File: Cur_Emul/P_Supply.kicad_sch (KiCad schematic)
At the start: 47 parts, among them J31 Conn_01x02_Pin, J49 Conn_01x04_Pin, J50 Conn_01x04_Pin, J51 Conn_01x02_Pin, J52 Conn_01x02_Pin, J53 Conn_01x02_Pin, J54 Conn_01x02_Pin, J55 Conn_01x02_Pin, U13 LM317_SOT-223, U15 LM7812_TO220, U7 LM317_SOT-223

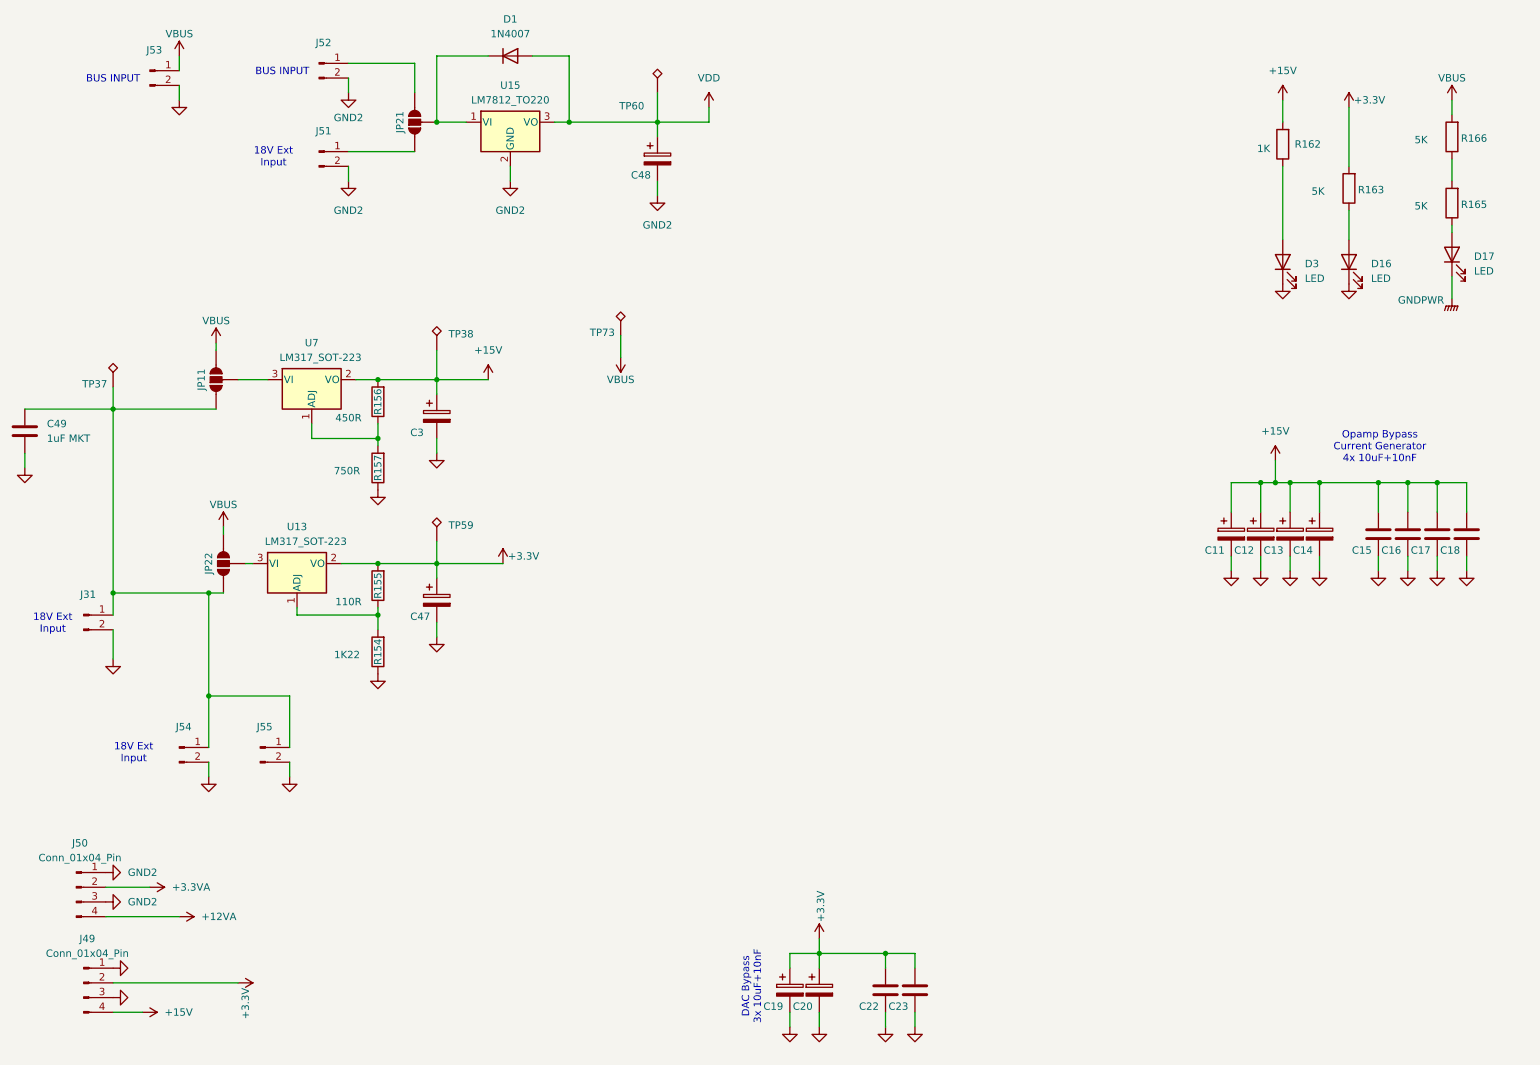
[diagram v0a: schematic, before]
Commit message: updates4
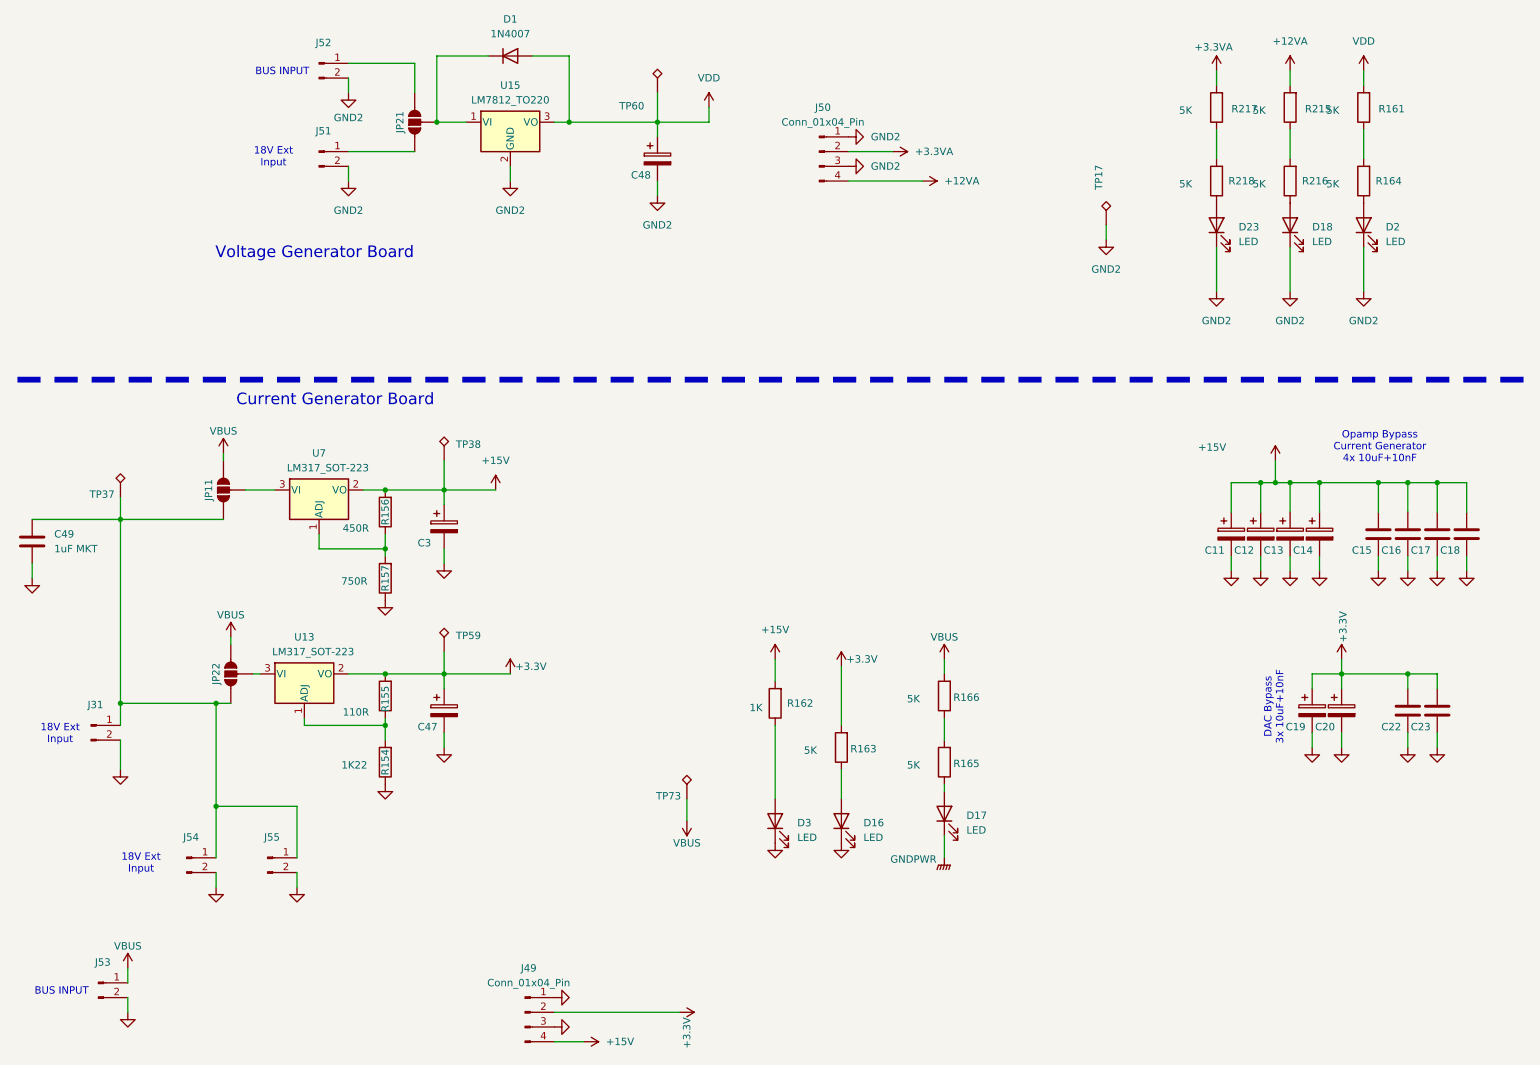
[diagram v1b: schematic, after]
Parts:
- added D18, D2, D23: LED, LED_SMD:LED_0805_2012Metric_Pad1.15x1.40mm_HandSolder, symbol Device:LED
- added R161, R164, R215, R216, R217, R218: 5K, Resistor_SMD:R_0805_2012Metric_Pad1.20x1.40mm_HandSolder, symbol Device:R
- added TP17: TestPoint_Alt, TestPoint:TestPoint_Loop_D1.80mm_Drill1.0mm_Beaded, symbol Connector:TestPoint_Alt
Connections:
- net +12VA: now also R215.2
- net +3.3VA: now also R217.2
- net GND2: now also D18.1 (K), D2.1 (K), D23.1 (K), TP17.1
- net VDD: now also R161.2
- new net: D23.2 (A), R218.1
- new net: R217.1, R218.2
- new net: D18.2 (A), R216.1
- new net: R215.1, R216.2
- new net: R161.1, R164.2
- new net: D2.2 (A), R164.1
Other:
- note added: "Current Generator Board"
- note added: "Voltage Generator Board"
- moved on the sheet: C19, C20, C22, C23, C3, C47, C49, D16, D17, D3, J31, J49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
